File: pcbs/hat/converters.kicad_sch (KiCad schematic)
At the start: 13 parts, among them U18 ADS7828, U19 ADS7828, U20 ADS7828, U21 LM3480-IM3-5.0

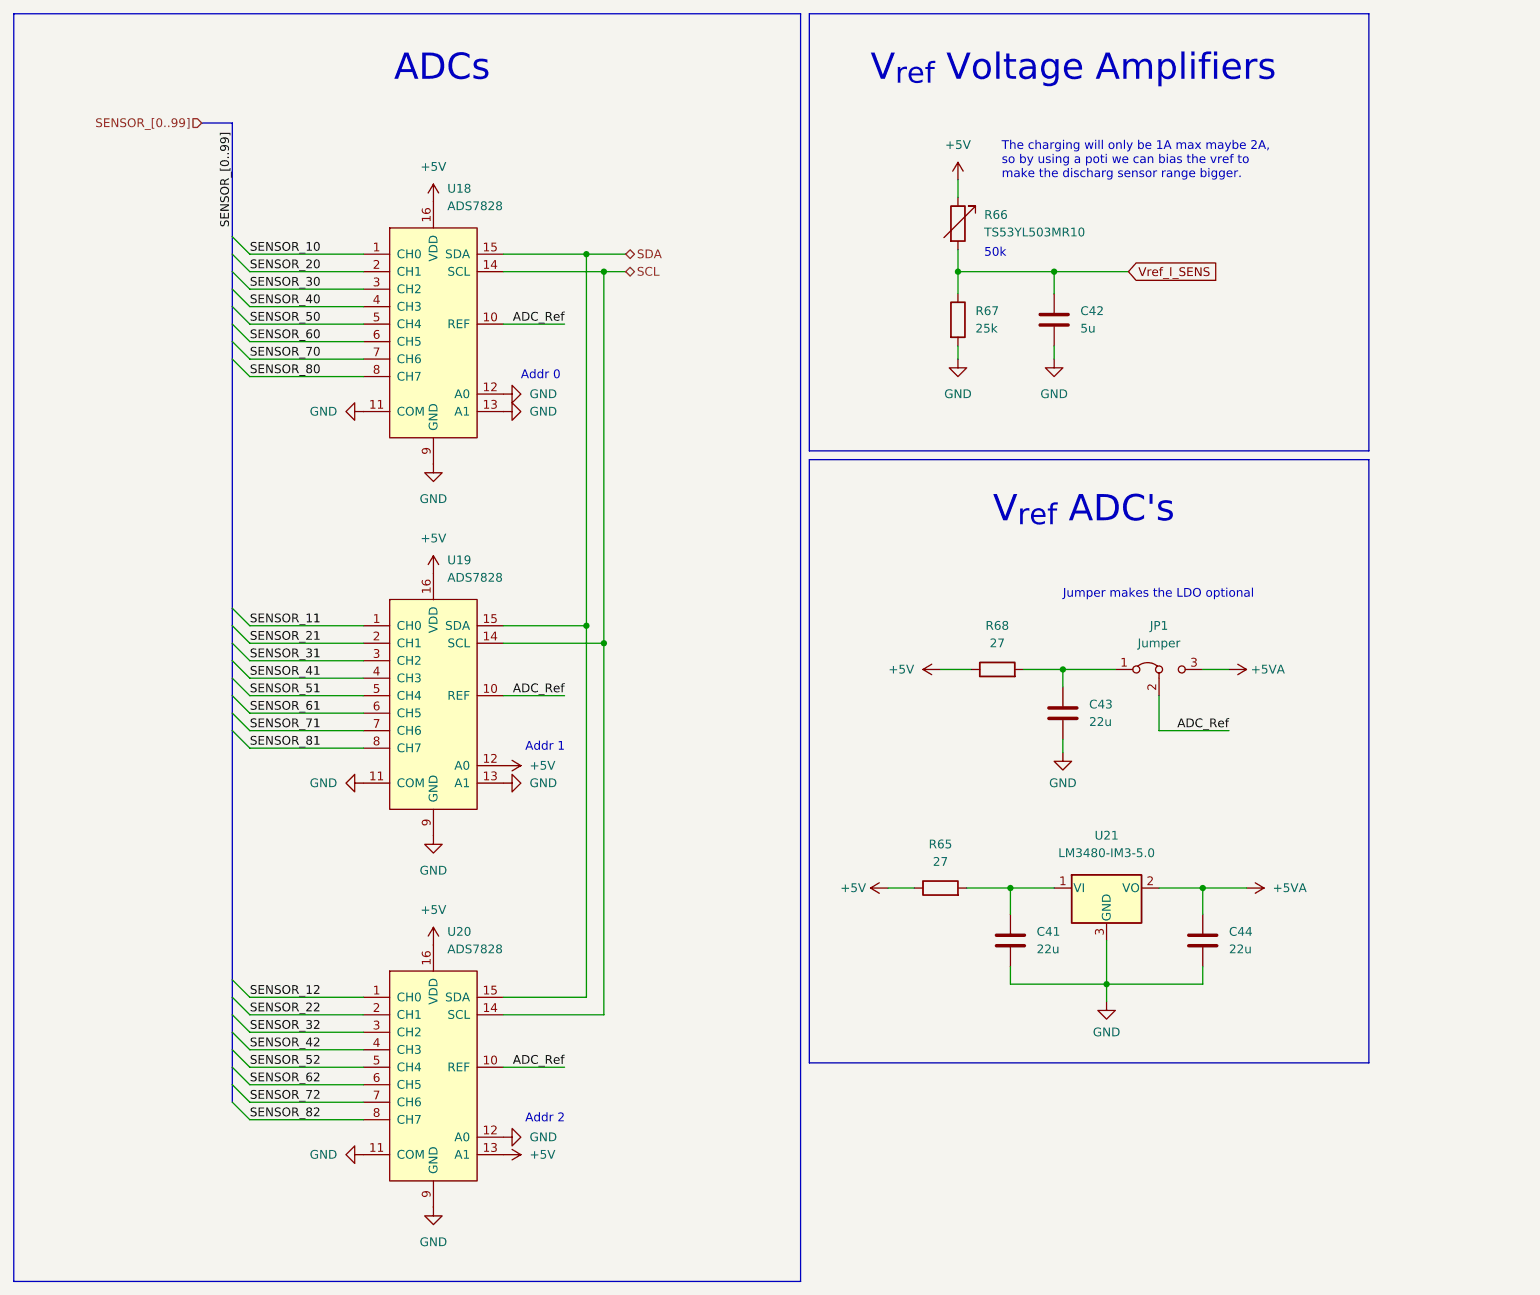
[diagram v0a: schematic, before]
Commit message: few little change
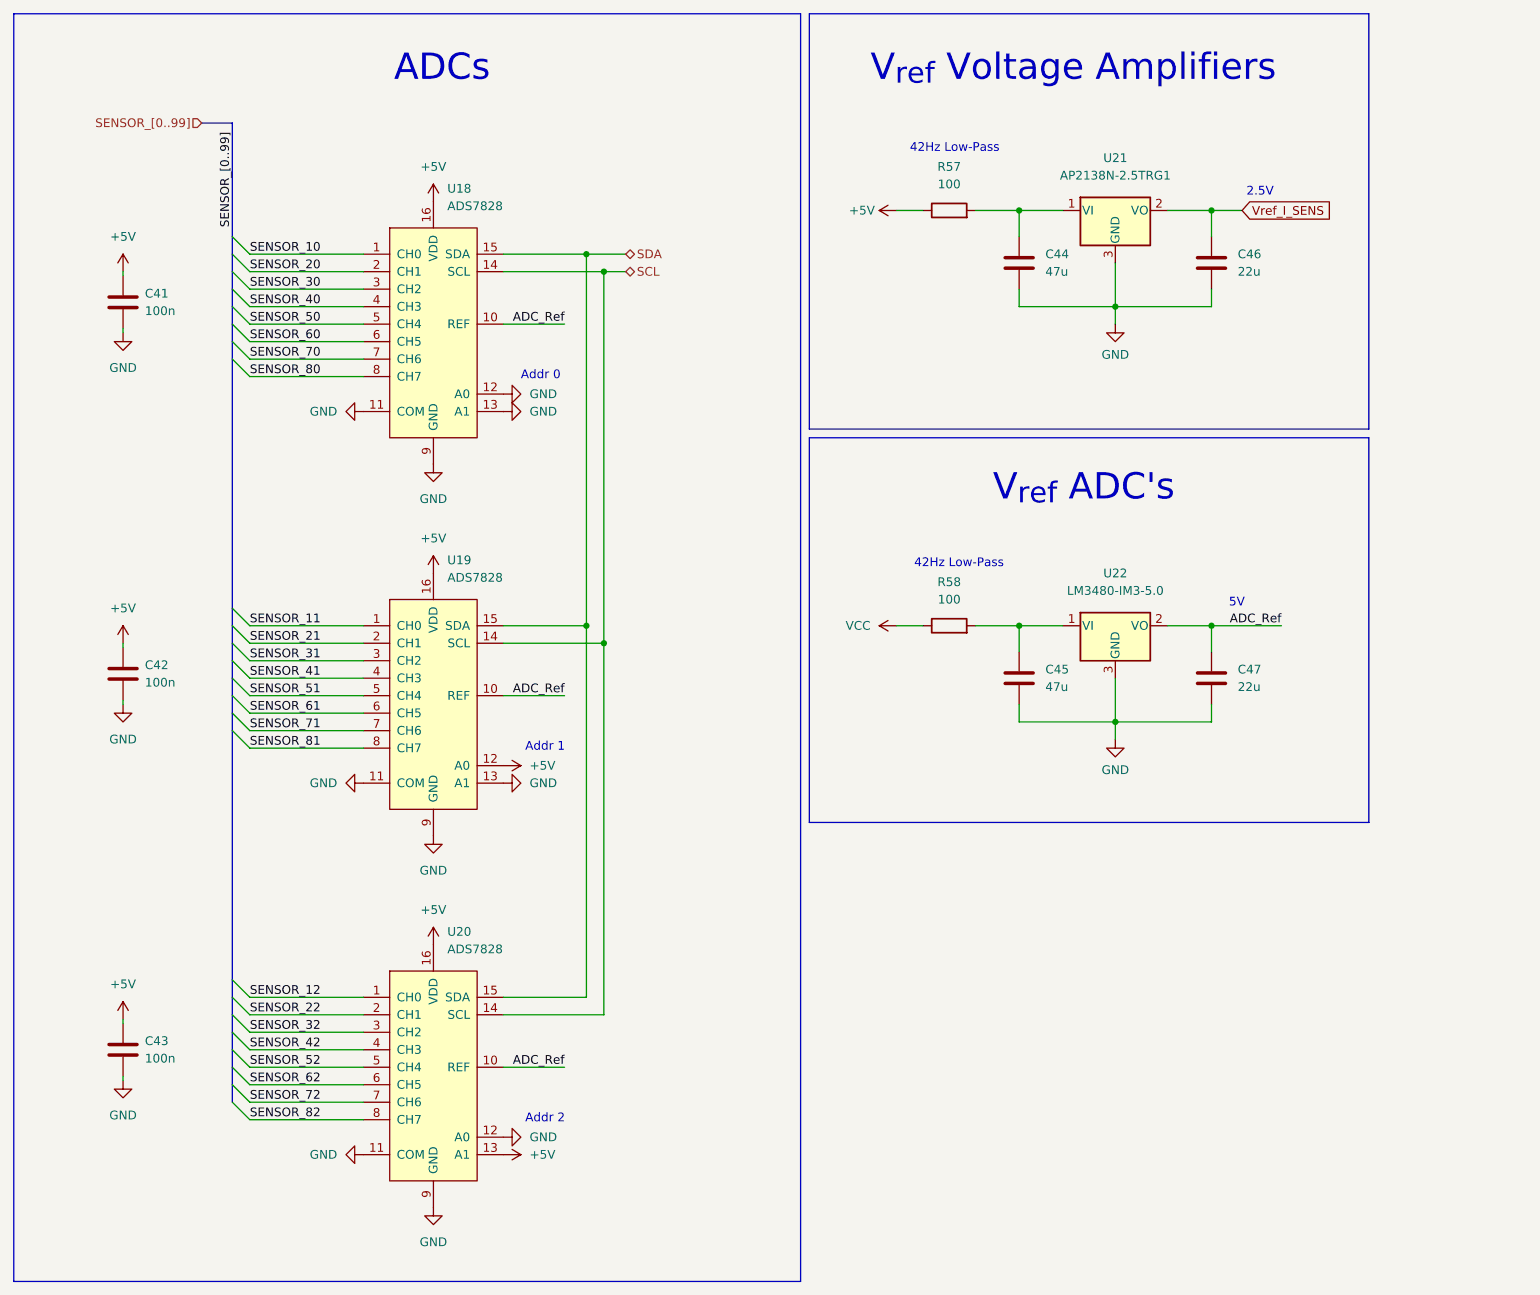
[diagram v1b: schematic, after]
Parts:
- removed JP1: Jumper, Connector_PinHeader_2.54mm:PinHeader_1x03_P2.54mm_Vertical, symbol Jumper:Jumper_3_Bridged12
- removed R66: TS53YL503MR10, Potentiometer_SMD:Potentiometer_Vishay_TS53YL_Vertical, symbol Device:R_Variable
- removed R67: 25k, Resistor_SMD:R_0805_2012Metric, symbol Device:R
- removed R68: 27, Resistor_SMD:R_0603_1608Metric, symbol Device:R
- added C44, C45: 47u, Capacitor_SMD:C_1206_3216Metric, symbol Device:C
- added C46: 22u, Capacitor_SMD:C_1206_3216Metric, symbol Device:C
- added R57: 100, Resistor_SMD:R_0603_1608Metric, symbol Device:R
- added U21: AP2138N-2.5TRG1, Package_TO_SOT_SMD:SOT-23, symbol Regulator_Linear:AP7384-70SA
- C41, C43: value 22u -> 100n; footprint Capacitor_SMD:C_1206_3216Metric -> (none)
- C42: value 5u -> 100n
- R58: renamed from R65; value 27 -> 100
- renumbered C44 to C47, U21 to U22
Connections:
- net +5VA is gone; now on net ADC_Ref: C47.2, U22.2 (VO)
- net +5V: now also C41.1, C42.1, C43.1, R57.1; no longer R58.1
- net GND: now also C41.2, C43.2, C44.1, C45.1, C46.1, U21.3 (GND); no longer C41.1, C43.1
- net Vref_I_SENS: now also C46.2, U21.2 (VO); no longer C42.1
- net at R58.2, U22.1 (VI): now also C45.2; no longer C41.2
- new net: C44.2, R57.2, U21.1 (VI)
- new net VCC: R58.1
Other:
- note added: "2.5V"
- note added: "42Hz Low-Pass"
- note added: "5V"
- note removed: "50k"
- note removed: "Jumper makes the LDO optional"
- note removed: "The charging will only be 1A max maybe 2A, so by using a poti we can bias the vref to make the discharg sensor range bigger."
- moved on the sheet: C47, R58, U22
